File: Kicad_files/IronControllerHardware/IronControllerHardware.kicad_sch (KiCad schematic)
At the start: 16 parts

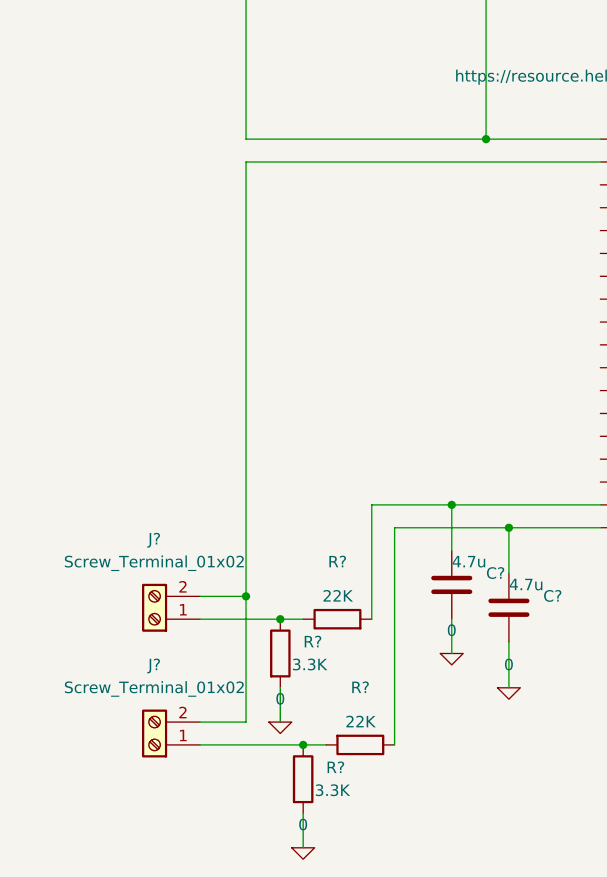
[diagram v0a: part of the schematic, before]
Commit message: update schematics
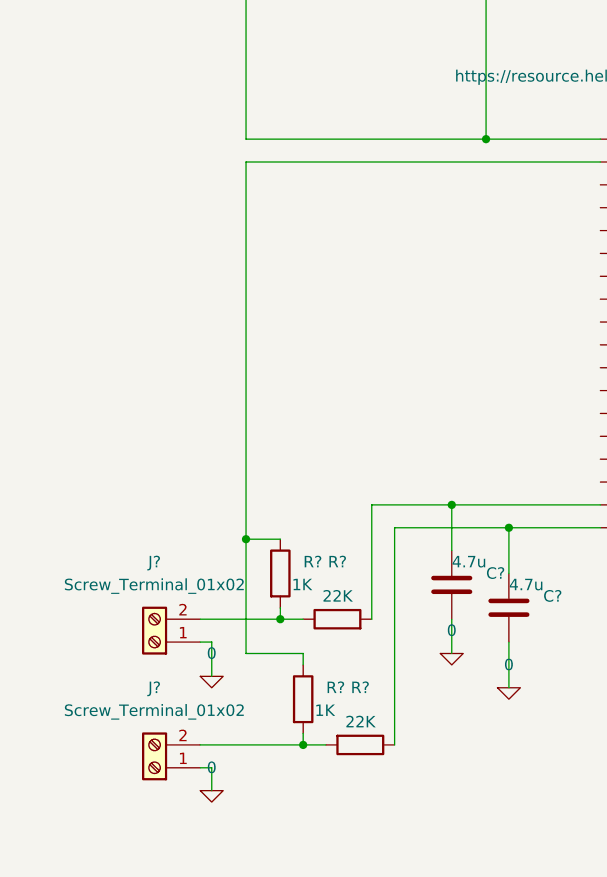
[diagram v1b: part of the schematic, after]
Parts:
- R? (x2): value 3.3K -> 1K
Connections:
- net 0: now also J?.1 (Pin_1), J?.1 (Pin_1); no longer R?.2, R?.2
- new net: R?.1, R?.1, U?.9 (3.3)
- new net: J?.2 (Pin_2), R?.2, R?.2
- new net: J?.2 (Pin_2), R?.1, R?.2
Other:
- moved on the sheet: J?, R?
